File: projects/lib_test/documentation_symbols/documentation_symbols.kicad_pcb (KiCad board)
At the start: 2 copper layers, 100 x 100 mm, 1 part

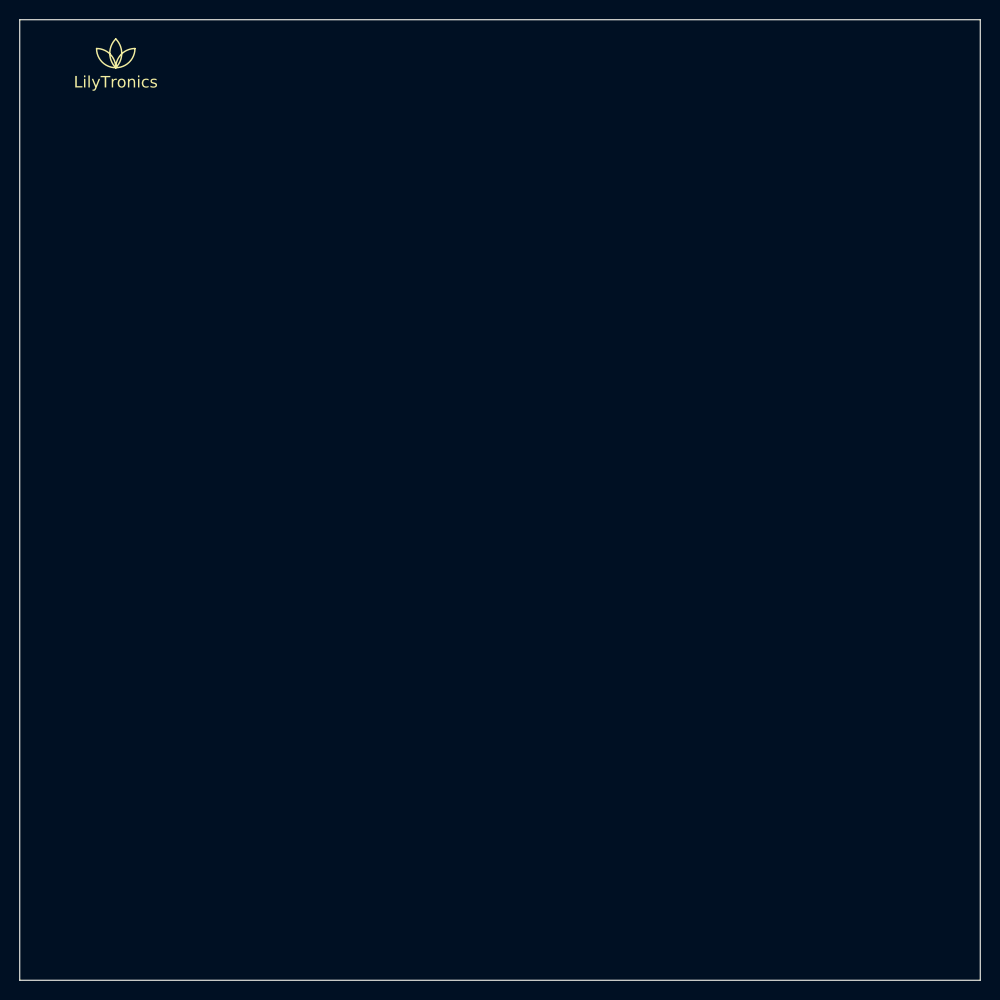
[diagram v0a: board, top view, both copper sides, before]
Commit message: updated test projects
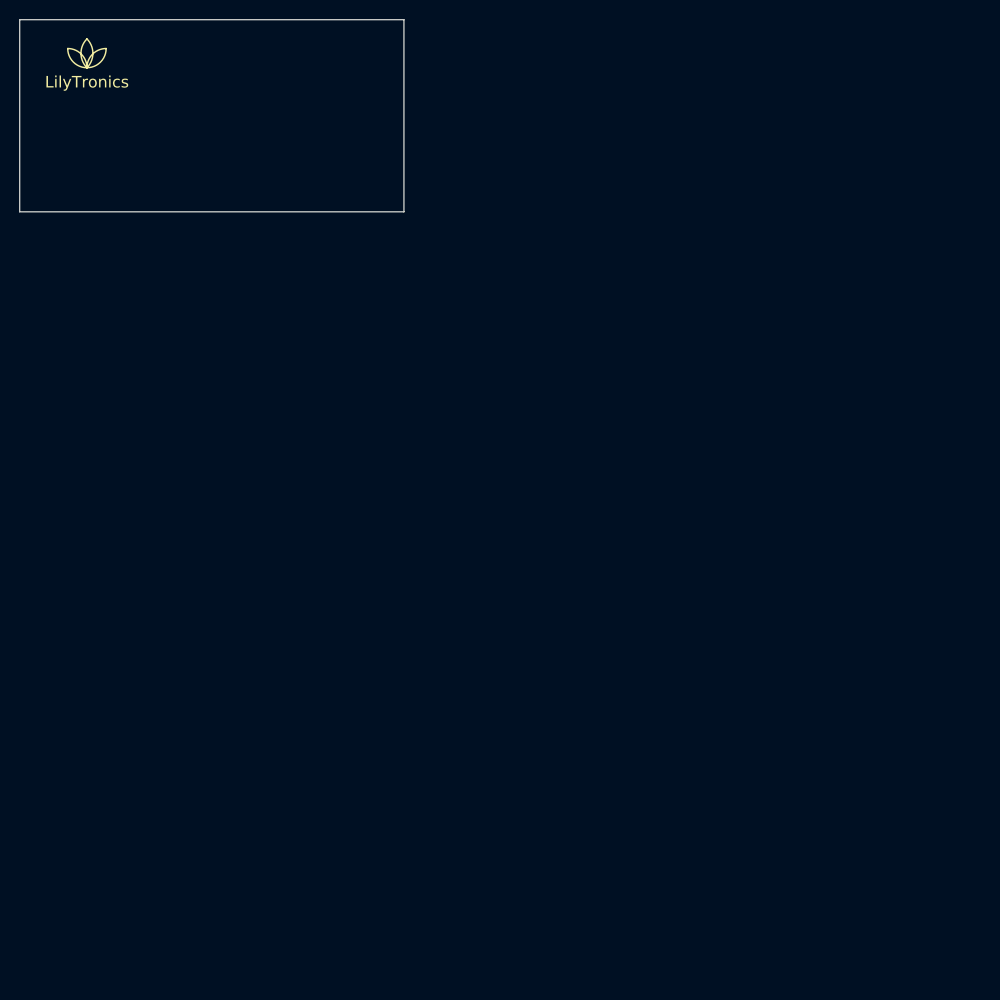
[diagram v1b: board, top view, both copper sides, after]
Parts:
- moved DOC1001 3.00 mm to (107.0, 55.0)
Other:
- board size 100 x 100 mm -> 40 x 20 mm
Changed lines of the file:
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@@
 (kicad_pcb
-	(version 20240108)
+	(version 20241229)
 	(generator "pcbnew")
-	(generator_version "8.0")
+	(generator_version "9.0")
 	(general
 		(thickness 1.6)
@@
 	(title_block
 		(title "Documentation symbols")
-		(date "2025-02-08")
+		(date "2025-05-24")
 		(rev "1")
 		(comment 1 "-")
@@
 	(layers
 		(0 "F.Cu" signal)
-		(31 "B.Cu" signal)
-		(34 "B.Paste" user)
-		(35 "F.Paste" user)
-		(36 "B.SilkS" user "B.Silkscreen")
-		(37 "F.SilkS" user "F.Silkscreen")
-		(38 "B.Mask" user)
-		(39 "F.Mask" user)
-		(40 "Dwgs.User" user "User.Drawings")
-		(41 "Cmts.User" user "User.Comments")
-		(44 "Edge.Cuts" user)
-		(45 "Margin" user)
-		(46 "B.CrtYd" user "B.Courtyard")
-		(47 "F.CrtYd" user "F.Courtyard")
-		(48 "B.Fab" user)
-		(49 "F.Fab" user)
+		(2 "B.Cu" signal)
+		(13 "F.Paste" user)
+		(15 "B.Paste" user)
+		(5 "F.SilkS" user "F.Silkscreen")
+		(7 "B.SilkS" user "B.Silkscreen")
+		(1 "F.Mask" user)
+		(3 "B.Mask" user)
+		(17 "Dwgs.User" user "User.Drawings")
+		(19 "Cmts.User" user "User.Comments")
+		(25 "Edge.Cuts" user)
+		(27 "Margin" user)
+		(31 "F.CrtYd" user "F.Courtyard")
+		(29 "B.CrtYd" user "B.Courtyard")
+		(35 "F.Fab" user)
+		(33 "B.Fab" user)
 	)
 	(setup
@@
 		(pad_to_mask_clearance 0)
 		(allow_soldermask_bridges_in_footprints no)
+		(tenting front back)
 		(pcbplotparams
-			(layerselection 0x00010fc_ffffffff)
-			(plot_on_all_layers_selection 0x0000000_00000000)
+			(layerselection 0x00000000_00000000_55555555_5755f5ff)
+			(plot_on_all_layers_selection 0x00000000_00000000_00000000_00000000)
 			(disableapertmacros no)
 			(usegerberextensions no)
@@
 			(svgprecision 6)
 			(plotframeref no)
-			(viasonmask no)
 			(mode 1)
 			(useauxorigin no)
@@
 			(pdf_front_fp_property_popups yes)
 			(pdf_back_fp_property_popups yes)
+			(pdf_metadata yes)
+			(pdf_single_document no)
 			(dxfpolygonmode yes)
 			(dxfimperialunits yes)
@@
 			(psnegative no)
 			(psa4output no)
-			(plotreference yes)
-			(plotvalue yes)
-			(plotfptext yes)
-			(plotinvisibletext no)
+			(plot_black_and_white yes)
 			(sketchpadsonfab no)
+			(plotpadnumbers no)
+			(hidednponfab no)
+			(sketchdnponfab yes)
+			(crossoutdnponfab yes)
 			(subtractmaskfromsilk no)
 			(outputformat 1)
@@
 	(footprint "lily_footprints:logo_lilytronics"
 		(layer "F.Cu")
-		(at 110 55)
+		(at 107 55)
 		(property "Reference" "DOC1001"
 			(at 0 -0.000002 0)
@@
 			)
 		)
-		(property "Footprint" "lily_footprints:logo_lilytronics"
+		(property "Datasheet" ""
 			(at 0 0 0)
 			(unlocked yes)
@@
 			)
 		)
-		(property "Datasheet" ""
+		(property "Description" ""
 			(at 0 0 0)
 			(unlocked yes)
@@
 			)
 		)
-		(property "Description" ""
-			(at 0 0 0)
-			(unlocked yes)
-			(layer "F.Fab")
-			(hide yes)
-			(effects
-				(font
-					(size 1.27 1.27)
-					(thickness 0.15)
-				)
-			)
-		)
 		(property "Revision" "1"
 			(at 0 0 0)
@@
 			)
 		)
-		(sheetname "Root")
+		(sheetname "/")
 		(sheetfile "documentation_symbols.kicad_sch")
 		(attr exclude_from_pos_files exclude_from_bom allow_missing_courtyard)
@@
 			)
 		)
-		(fp_text user "${REFERENCE}"
-			(at 0.000001 -0.000001 0)
-			(layer "F.Fab")
-			(hide yes)
-			(effects
-				(font
-					(size 0.5 0.5)
-					(thickness 0.1)
-				)
-			)
-		)
+		(embedded_fonts no)
 	)
 	(gr_rect
 		(start 100 50)
-		(end 200 150)
+		(end 140 70)
 		(stroke
 			(width 0.1)
 			(type default)
 		)
-		(fill none)
+		(fill no)
 		(layer "Edge.Cuts")
 	)
+	(embedded_fonts no)
 )
